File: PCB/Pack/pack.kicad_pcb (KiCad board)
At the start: 2 copper layers, 100 x 100 mm, 43 parts, among them J1 Conn_01x01, J2 Conn_01x01, J3 Conn_01x01, J4 Conn_01x01, J5 Conn_01x01, J6 Conn_01x01, J7 Conn_01x02, J8 Conn_01x02

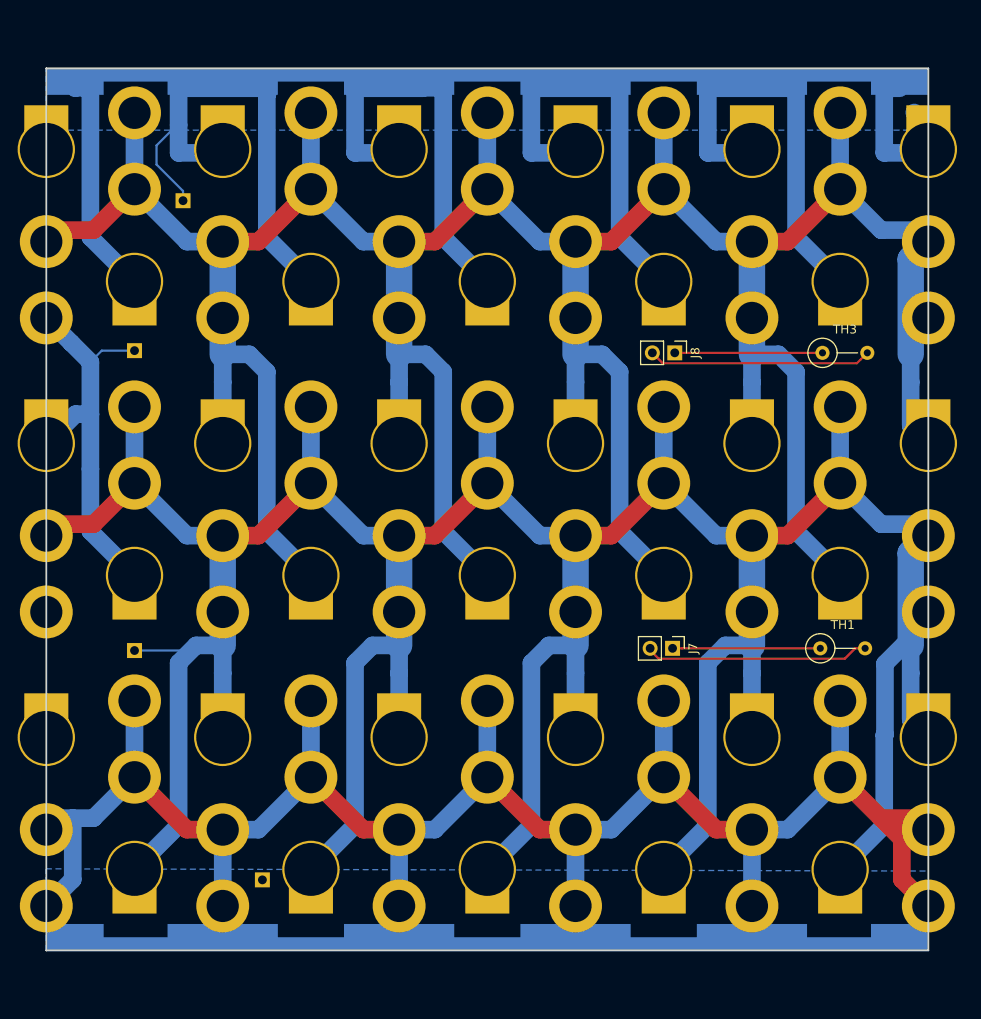
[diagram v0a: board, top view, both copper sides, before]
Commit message: small change
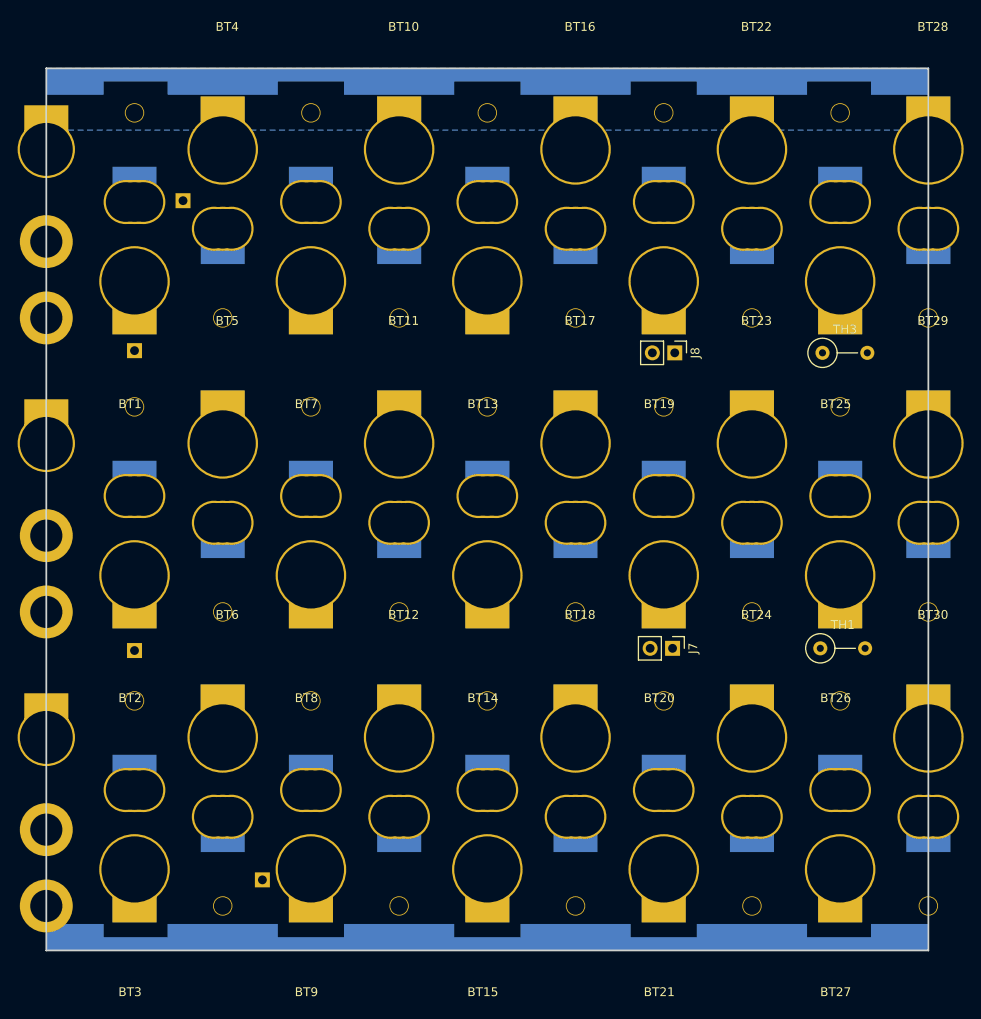
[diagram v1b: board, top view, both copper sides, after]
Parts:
- BT1, BT10, BT11, BT12, BT13, BT14, BT15, BT16, BT17, BT18, BT19, BT2, BT20, BT21, BT22, BT23, BT24, BT25, BT26, BT27, BT28, BT29, BT3, BT30, BT4, BT5, BT6, BT7, BT8, BT9: footprint ENNOID:Battery -> ENNOID:18650
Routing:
- net Net-(BT1-Pad2): track 445.1 -> 0.00 mm
- net Net-(BT11-Pad2): track 440.3 -> 0.00 mm
- net Net-(BT1-Pad1): track 423.3 -> 0.00 mm
- net Net-(BT12-Pad2): track 229.7 -> 0.00 mm
- net Net-(J7-Pad2): track 25.5 -> 0.00 mm
- net Net-(J8-Pad2): track 25.3 -> 0.00 mm
- net Net-(J8-Pad1): track 16.8 -> 0.00 mm
- net Net-(J7-Pad1): track 16.8 -> 0.00 mm
- removed copper zone on B.Cu, net Net-(BT12-Pad2)
